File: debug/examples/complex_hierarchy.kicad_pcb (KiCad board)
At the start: 2 copper layers, 100.7 x 80 mm, 68 parts, among them P1 CONN_2, P2 CONN_2, P3 CONN_2, P4 CONN_2, P5 CONN_2, P6 CONN_2, Q1 MPSA92, Q2 MPSA42, Q3 MPSA92, Q4 MPSA42, Q5 MPSA92, Q6 MPSA42, Q7 MPSA92, Q8 MPSA42, U1 ICL7660, U2 78L05, U3 LM358N, U4 LM358N

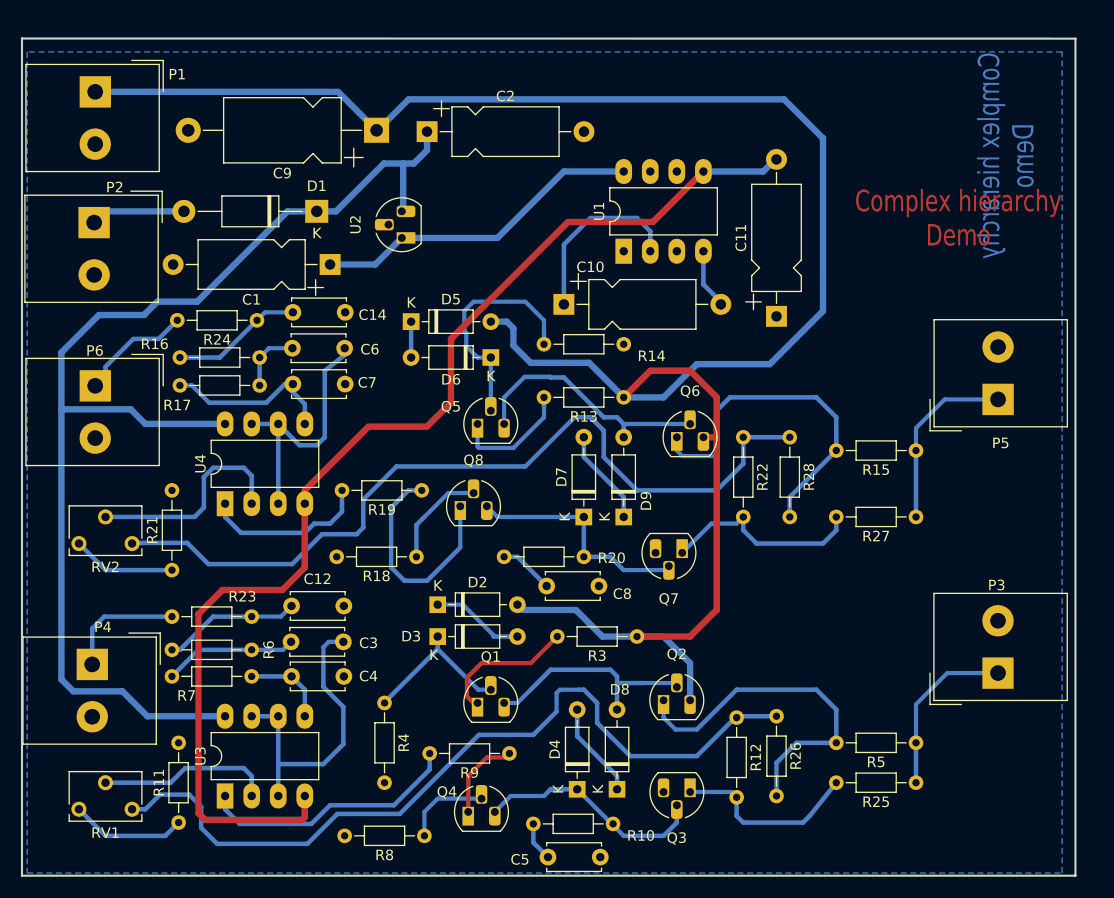
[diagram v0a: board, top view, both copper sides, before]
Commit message: Update example
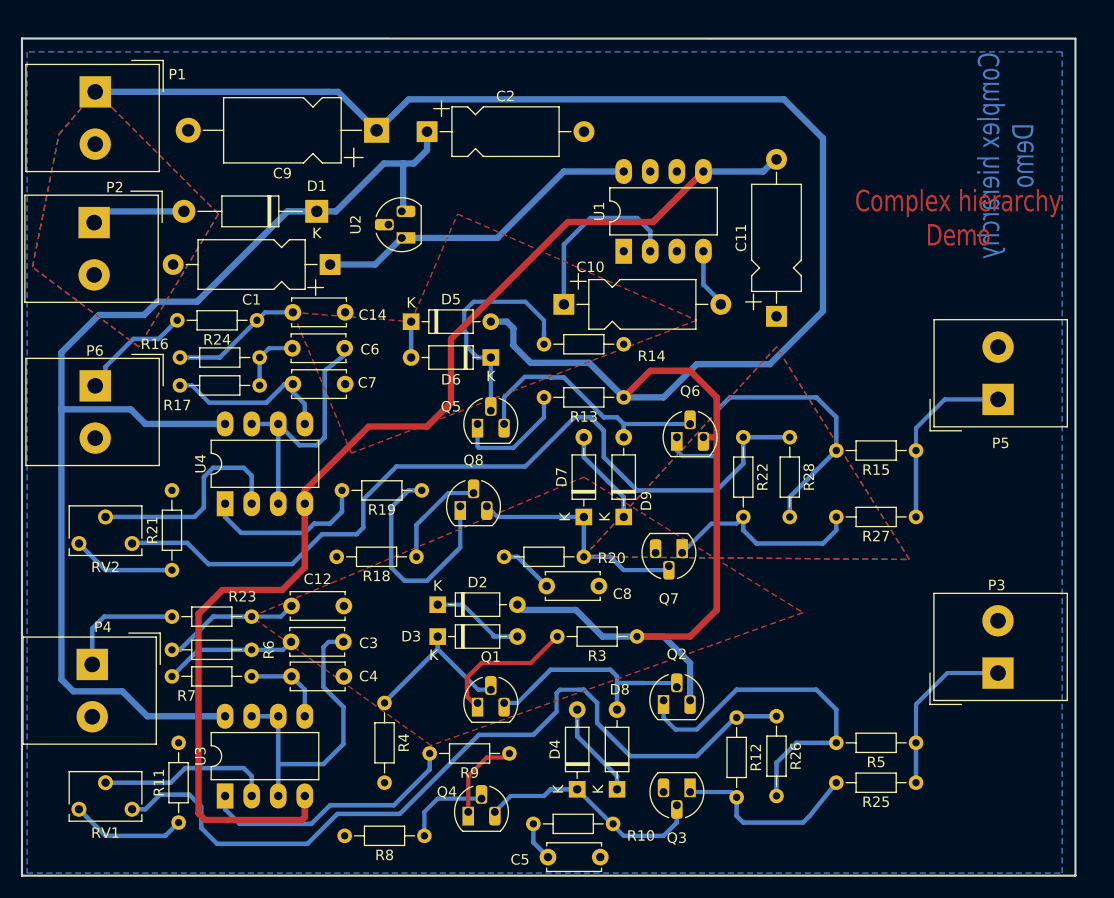
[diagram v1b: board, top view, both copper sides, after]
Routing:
- added copper zone on F.Cu, net +12V
- added copper zone on B.Cu, net /ampli_ht_horizontal/S_OUT+
- added copper zone on F.Cu, net /ampli_ht_horizontal/S_OUT+
- added copper zone on B.Cu, net /ampli_ht_vertical/PIEZO_IN
- added copper zone on F.Cu, net /ampli_ht_vertical/PIEZO_IN
- added copper zone on F.Cu, net /ampli_ht_vertical/Vpil_0_3,3V
- added copper zone on In1.Cu, net /ampli_ht_vertical/Vpil_0_3,3V
- added copper zone on In2.Cu, net /ampli_ht_vertical/Vpil_0_3,3V
- added copper zone on In3.Cu, net /ampli_ht_vertical/Vpil_0_3,3V
- added copper zone on In4.Cu, net /ampli_ht_vertical/Vpil_0_3,3V
- added copper zone on In5.Cu, net /ampli_ht_vertical/Vpil_0_3,3V
- added copper zone on In6.Cu, net /ampli_ht_vertical/Vpil_0_3,3V
- added copper zone on In7.Cu, net /ampli_ht_vertical/Vpil_0_3,3V
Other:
- copper layers 2 -> 20
